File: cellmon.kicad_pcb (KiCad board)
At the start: 2 copper layers, 32 x 25 mm, 13 parts, among them J1 Conn_01x02_Male, J2 Conn_01x02_Male, J3 Conn_01x06, J4 Conn_01x02_Male, U1 ATtiny85V-10S, U2 6N136

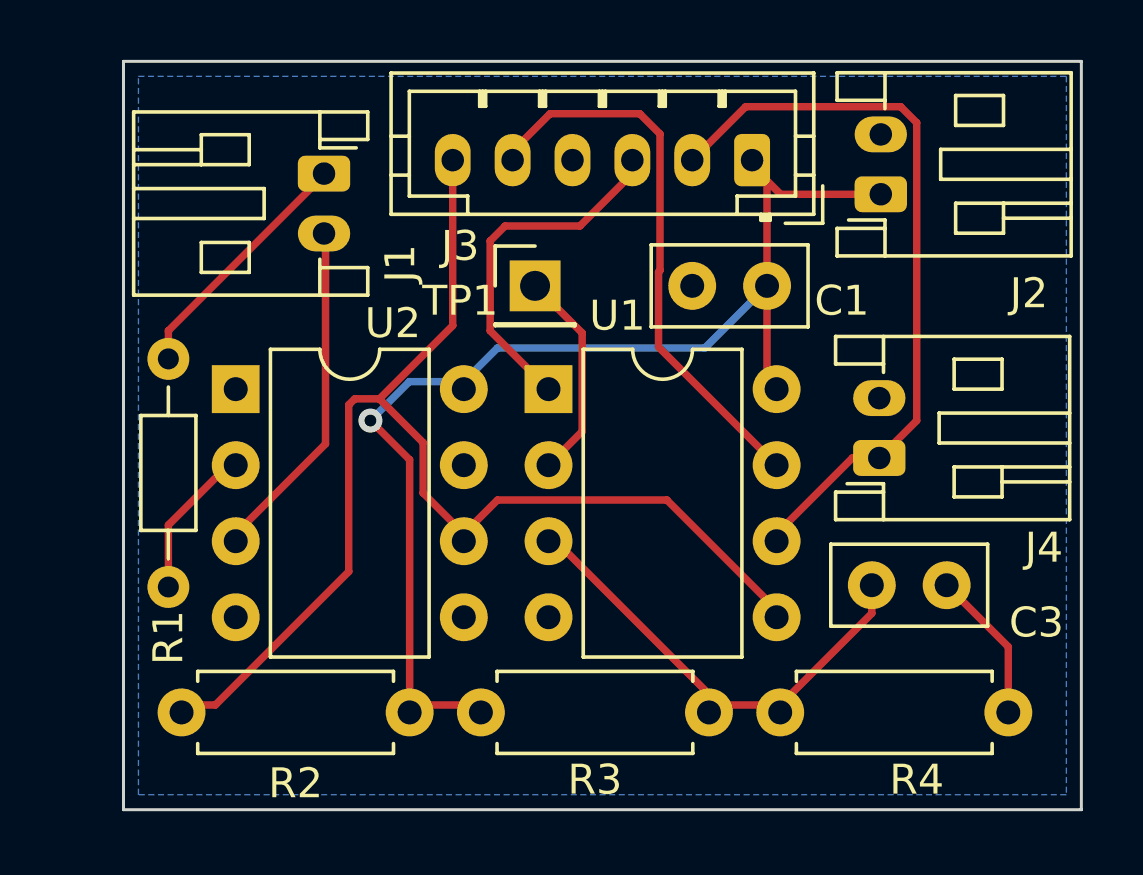
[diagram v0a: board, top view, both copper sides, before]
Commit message: Update to R2 PCB
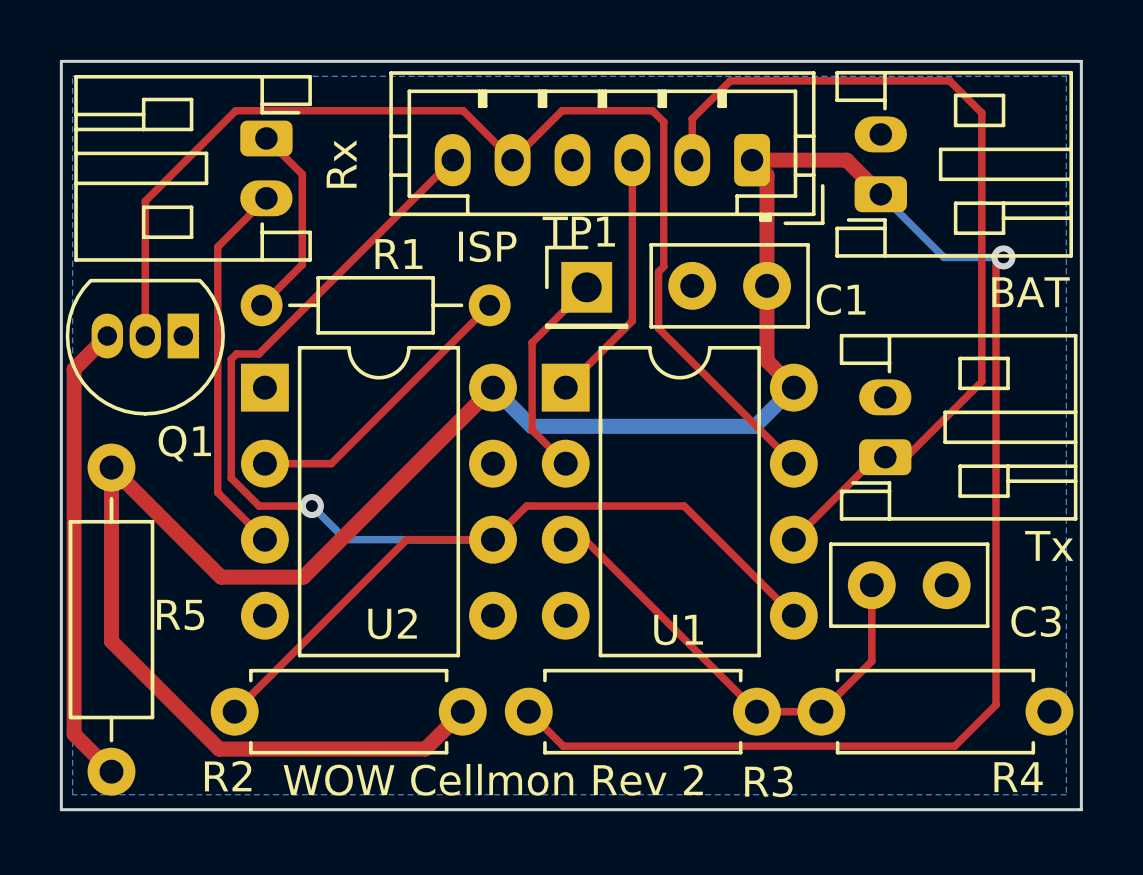
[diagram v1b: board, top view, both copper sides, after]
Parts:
- added Q1: 2N7000, Package_TO_SOT_THT:TO-92_Inline, F.Cu at (122.0, 69.2)
- added R5: 20R 1 watt, Resistor_THT:R_Axial_DIN0207_L6.3mm_D2.5mm_P10.16mm_Horizontal, F.Cu at (119.6, 83.7)
- R1: value 2K2 -> 220R
- R2: value 10K -> 4K7
- moved R1 3.59 mm to (124.6, 68.2), turned to 0 degrees
- moved Rx 2.26 mm to (124.8, 62.6)
- moved R2 1.78 mm to (131.3, 81.7)
- moved TP1 1.73 mm to (135.5, 67.5)
- moved R3 1.60 mm to (133.5, 81.7)
- moved R4 1.38 mm to (143.3, 81.7)
- moved U2 0.98 mm to (124.7, 70.9)
- moved U1 0.58 mm to (134.8, 70.9)
- moved Tx 0.20 mm to (145.4, 73.2)
- renumbered J2 to BAT, J3 to ISP, J1 to Rx, J4 to Tx
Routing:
- net VCC: track 39.0 -> 97.3 mm
- net /SCK: track 18.7 -> 38.0 mm
- net Net-(Q1-Pad3): track 0.00 -> 15.5 mm
- net /Rx/MOSI: track 41.2 -> 46.8 mm, vias 0 -> 1
- net GND: track 4.85 -> 0.00 mm
- net /Tx/MISO: track 24.7 -> 29.5 mm
- net Net-(R1-Pad2): track 5.25 -> 9.70 mm
- net /RST: track 11.9 -> 8.52 mm
- net Net-(Rx1-Pad1): track 8.36 -> 6.63 mm
- net Net-(Rx1-Pad2): track 11.3 -> 12.7 mm
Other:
- board size 32 x 25 mm -> 34.1 x 25 mm
- board text added: "WOW Cellmon Rev 2"

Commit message: R2 PCB
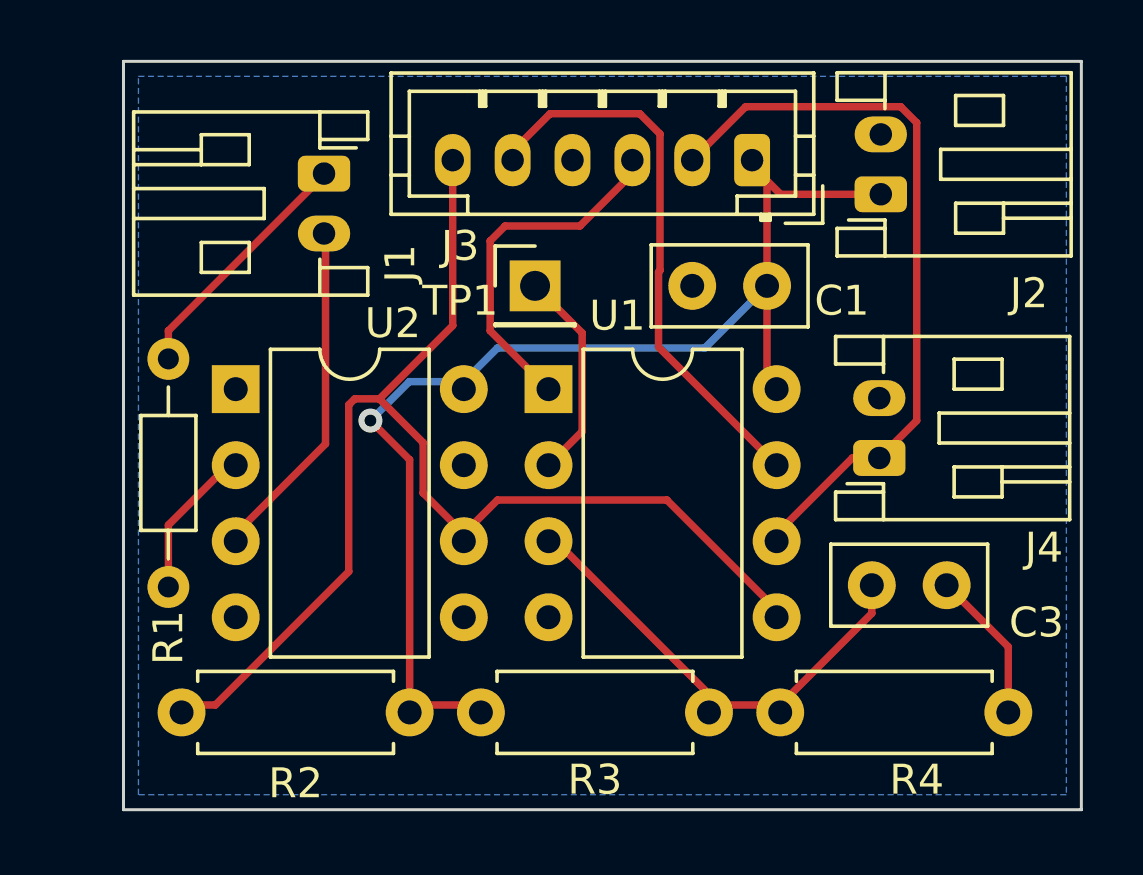
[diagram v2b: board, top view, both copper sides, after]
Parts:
- removed Q1: 2N7000, Package_TO_SOT_THT:TO-92_Inline
- removed R5: 20R 1 watt, Resistor_THT:R_Axial_DIN0207_L6.3mm_D2.5mm_P10.16mm_Horizontal
- R1: value 220R -> 2K2
- R2: value 4K7 -> 10K
- moved R1 3.59 mm to (121.5, 69.9), turned to -90 degrees
- moved J1 2.26 mm to (126.7, 63.8)
- moved R2 1.78 mm to (129.6, 81.8)
- moved TP1 1.73 mm to (133.8, 67.5)
- moved R3 1.60 mm to (131.9, 81.8)
- moved R4 1.38 mm to (141.9, 81.8)
- moved U2 0.98 mm to (123.8, 71.0)
- moved U1 0.58 mm to (134.2, 71.0)
- moved J4 0.20 mm to (145.2, 73.2)
- renumbered Rx to J1, BAT to J2, ISP to J3, Tx to J4
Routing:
- net VCC: track 97.3 -> 39.0 mm
- net /SCK: track 38.0 -> 18.7 mm
- net Net-(Q1-Pad3): track 15.5 -> 0.00 mm
- net /Rx/MOSI: track 46.8 -> 41.2 mm, vias 1 -> 0
- net GND: track 0.00 -> 4.85 mm
- net /Tx/MISO: track 29.5 -> 24.7 mm
- net Net-(R1-Pad2): track 9.70 -> 5.25 mm
- net /RST: track 8.52 -> 11.9 mm
- net Net-(J1-Pad1): track 6.63 -> 8.36 mm
- net Net-(J1-Pad2): track 12.7 -> 11.3 mm
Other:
- board size 34.1 x 25 mm -> 32 x 25 mm
- board text removed: "WOW Cellmon Rev 2"
